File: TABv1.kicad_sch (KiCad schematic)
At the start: 41 parts, among them J10 Conn_UART_HOST, J11 Conn_UART_1, J12 Conn_UART_0, J13 Conn_ADC, J2 Conn_02x03_Row_Letter_Last, J3 Conn_02x03_Row_Letter_Last, J6 SWD, J8 Conn_SPI1, J9 Conn_SPI0, Q2 NMOS, SW2 RESET, U1 RP2350B-QFN80, Y1 12MHz

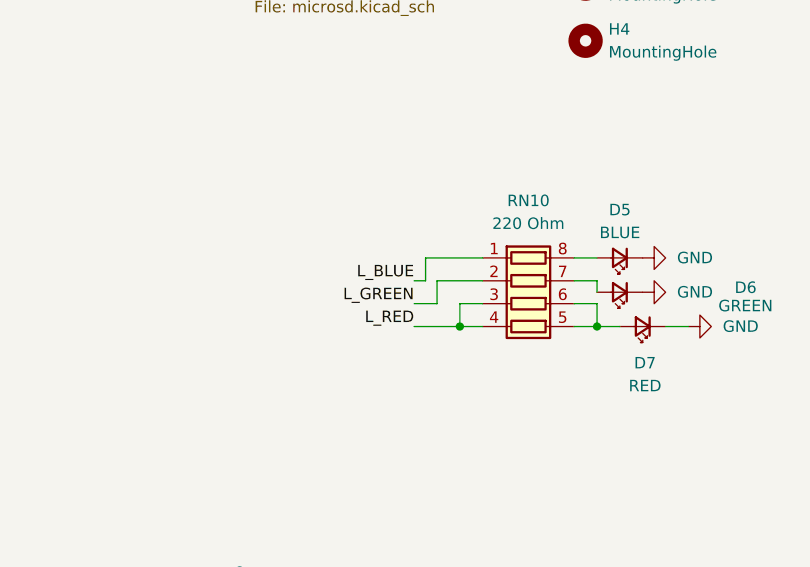
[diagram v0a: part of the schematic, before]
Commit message: Corrections
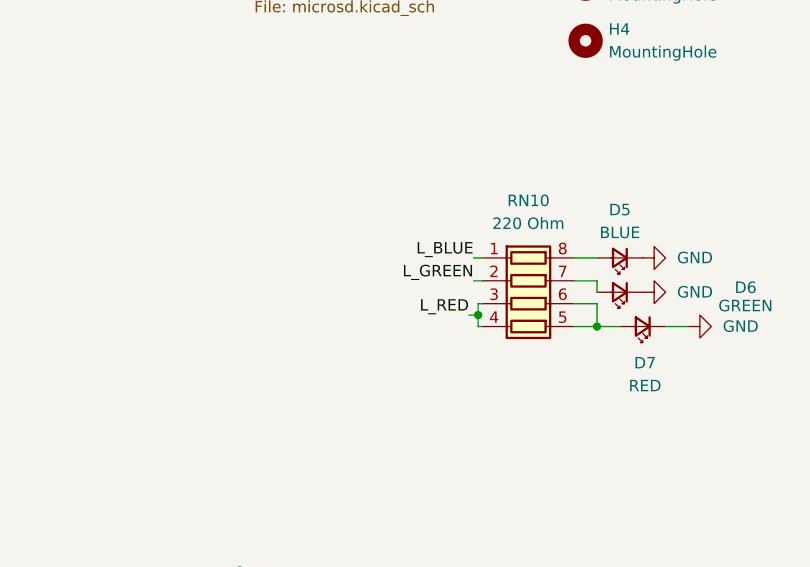
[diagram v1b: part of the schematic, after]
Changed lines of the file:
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@@
 	)
 	(junction
-		(at 351.79 194.31)
-		(diameter 0)
-		(color 0 0 0 0)
-	)
-	(junction
 		(at 336.55 237.49)
 		(diameter 0)
@@
 	)
 	(junction
+		(at 353.822 193.04)
+		(diameter 0)
+		(color 0 0 0 0)
+	)
+	(junction
 		(at 106.68 68.58)
 		(diameter 0)
@@
 	(wire
 		(pts
+			(xy 353.314 189.23) (xy 354.33 189.23)
+		)
+		(stroke
+			(width 0)
+			(type default)
+		)
+	)
+	(wire
+		(pts
 			(xy 217.17 107.95) (xy 232.41 107.95)
 		)
@@
 	(wire
 		(pts
+			(xy 352.806 193.04) (xy 353.822 193.04)
+		)
+		(stroke
+			(width 0)
+			(type default)
+		)
+	)
+	(wire
+		(pts
 			(xy 26.67 261.62) (xy 26.67 262.89)
 		)
@@
 	(wire
 		(pts
-			(xy 349.25 189.23) (xy 354.33 189.23)
-		)
-		(stroke
-			(width 0)
-			(type default)
-		)
-	)
-	(wire
-		(pts
 			(xy 55.88 85.09) (xy 77.47 85.09)
 		)
@@
 	(wire
 		(pts
-			(xy 346.71 194.31) (xy 351.79 194.31)
-		)
-		(stroke
-			(width 0)
-			(type default)
-		)
-	)
-	(wire
-		(pts
 			(xy 43.18 142.24) (xy 43.18 144.78)
 		)
@@
 		)
 	)
+	(wire
+		(pts
+			(xy 353.822 191.77) (xy 353.822 193.04)
+		)
+		(stroke
+			(width 0)
+			(type default)
+		)
+	)
 	(polyline
 		(pts
@@
 	(wire
 		(pts
-			(xy 351.79 194.31) (xy 354.33 194.31)
+			(xy 353.822 194.31) (xy 354.33 194.31)
 		)
 		(stroke
@@
 	(wire
 		(pts
-			(xy 354.33 191.77) (xy 351.79 191.77)
+			(xy 354.33 191.77) (xy 353.822 191.77)
 		)
 		(stroke
@@
 		)
 	)
-	(wire
-		(pts
-			(xy 347.98 186.69) (xy 354.33 186.69)
-		)
-		(stroke
-			(width 0)
-			(type default)
-		)
-	)
 	(polyline
 		(pts
@@
 	(wire
 		(pts
+			(xy 353.822 193.04) (xy 353.822 194.31)
+		)
+		(stroke
+			(width 0)
+			(type default)
+		)
+	)
+	(wire
+		(pts
 			(xy 147.32 96.52) (xy 166.37 96.52)
 		)
@@
 	(wire
 		(pts
-			(xy 347.98 189.23) (xy 347.98 186.69)
-		)
-		(stroke
-			(width 0)
-			(type default)
-		)
-	)
-	(wire
-		(pts
 			(xy 78.74 69.85) (xy 78.74 67.31)
 		)
@@
 		)
 	)
-	(wire
-		(pts
-			(xy 349.25 191.77) (xy 349.25 189.23)
-		)
-		(stroke
-			(width 0)
-			(type default)
-		)
-	)
 	(polyline
 		(pts
@@
 	(wire
 		(pts
-			(xy 346.71 189.23) (xy 347.98 189.23)
+			(xy 353.314 186.69) (xy 354.33 186.69)
 		)
 		(stroke
@@
 		)
 	)
-	(wire
-		(pts
-			(xy 351.79 191.77) (xy 351.79 194.31)
-		)
-		(stroke
-			(width 0)
-			(type default)
-		)
-	)
 	(bus
 		(pts
@@
 	(wire
 		(pts
-			(xy 346.71 191.77) (xy 349.25 191.77)
-		)
-		(stroke
-			(width 0)
-			(type default)
-		)
-	)
-	(wire
-		(pts
 			(xy 147.32 149.86) (xy 166.37 149.86)
 		)
@@
 	)
 	(label "L_GREEN"
-		(at 346.71 191.77 180)
+		(at 353.314 189.23 180)
 		(effects
 			(font
@@
 	)
 	(label "L_RED"
-		(at 346.71 194.31 180)
+		(at 352.806 193.04 180)
 		(effects
 			(font
@@
 	)
 	(label "L_BLUE"
-		(at 346.71 189.23 180)
+		(at 353.314 186.69 180)
 		(effects
 			(font
